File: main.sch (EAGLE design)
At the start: 5 parts, among them U1 ATMEGA328P_PDIP

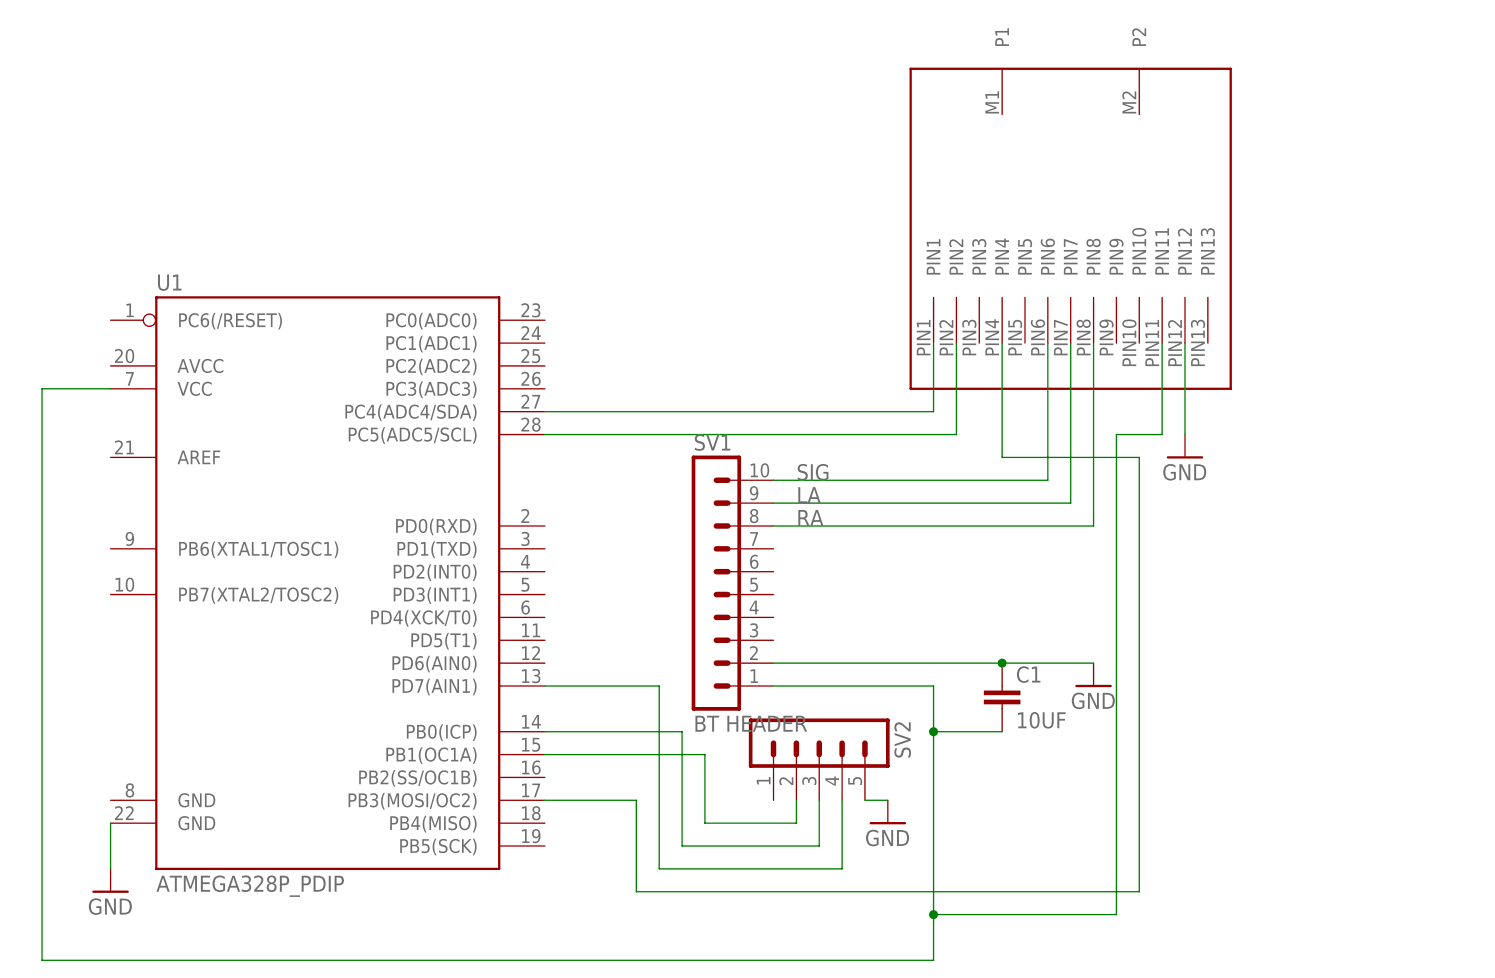
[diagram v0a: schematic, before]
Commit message: Added files via upload
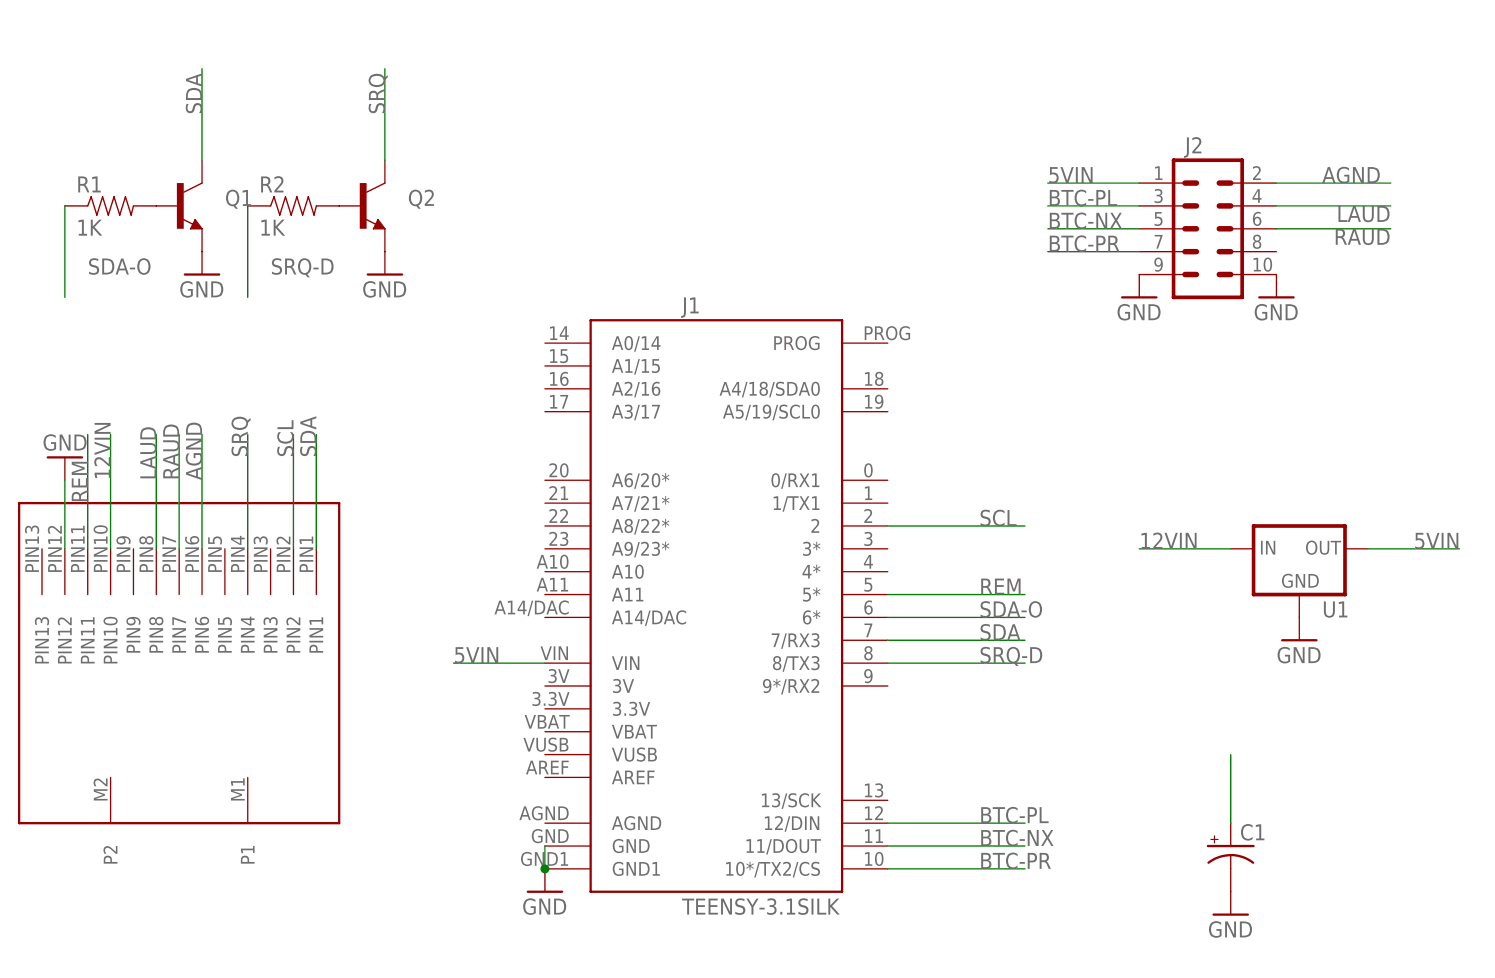
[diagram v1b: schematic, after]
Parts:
- removed SV1: BT HEADER, con-lstb:MA10-1
- removed SV2: (no value), con-lstb:MA05-1
- added J1: TEENSY-3.1SILK, SparkFun-Boards:TEENSY-3.1SILK
- added J2: (no value), SparkFun-Connectors:M05X2NO_SILK
- added Q1, Q2: (no value), SparkFun-DiscreteSemi:TRANSISTOR_NPN2N3904
- added R1, R2: 1K, SparkFun-Resistors:1KOHM-1/4W-1%(PTH)
- C1: value 10UF -> (none); device SparkFun-Capacitors:10UF10V10%(0805) -> SparkFun-Capacitors:10UF-25V-20%(PTH)
- U1: value ATMEGA328P_PDIP -> (none); device SparkFun-DigitalIC:ATMEGA328P_PDIP -> SparkFun-PowerIC:V_REG_78XX-TO-220
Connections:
- removed net LA: SV1.9, U$1.PIN7
- removed net N$10: SV2.3, U1.PB0(ICP)
- removed net N$11: SV2.2, U1.PB1(OC1A)
- removed net N$3: U$1.PIN4, U1.PB3(MOSI/OC2)
- removed net N$5: C1.2, SV1.1, U$1.PIN11, U1.VCC
- removed net N$9: SV2.4, U1.PD7(AIN1)
- removed net RA: SV1.8, U$1.PIN8
- removed net SIG: SV1.10, U$1.PIN6
- new net 12VIN: U$1.PIN10, U1.IN
- new net 5VIN: C1.+, J1.VIN, J2.1, U1.OUT
- new net AGND: J2.2, U$1.PIN6
- new net BTC-NX: J1.11/DOUT, J2.5
- new net BTC-PL: J1.12/DIN, J2.3
- new net BTC-PR: J1.10*/TX2/CS, J2.7
- new net LAUD: J2.4, U$1.PIN8
- new net RAUD: J2.6, U$1.PIN7
- new net REM: J1.5*, U$1.PIN11
- new net SCL: J1.2, U$1.PIN2
- new net SDA: J1.7/RX3, Q1.C, U$1.PIN1
- new net SDA-O: J1.6*, R1.1
- new net SRQ: Q2.C, U$1.PIN4
- new net SRQ-D: J1.8/TX3, R2.1
- net GND: now also C1.-, J1.GND, J1.GND1, J2.10, J2.9, Q1.E, Q2.E, U1.GND; no longer C1.1, SV1.2, SV2.5, U1.GND@2
- net N$1: now also Q1.B, R1.2; no longer U$1.PIN1, U1.PC4(ADC4/SDA)
- net N$2: now also Q2.B, R2.2; no longer U$1.PIN2, U1.PC5(ADC5/SCL)
